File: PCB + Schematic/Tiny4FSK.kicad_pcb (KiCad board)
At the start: 4 copper layers, 35.1 x 73.6 mm, 88 parts, among them J1 Power Ext, J2 GPIO, J3 I2C, J4 USB, J5 USB Breakout, J6 SPI, J7 USBC, J8 SWD, SW1 Power Switch, SW2 RST, U1 BME280, U2 ATGM336H, U3 TPS61200DRC, U4 ECS-327TXO-2012, U5 ATSAMD21G18A-A, U6 SI4063, U7 Linear Step-Down

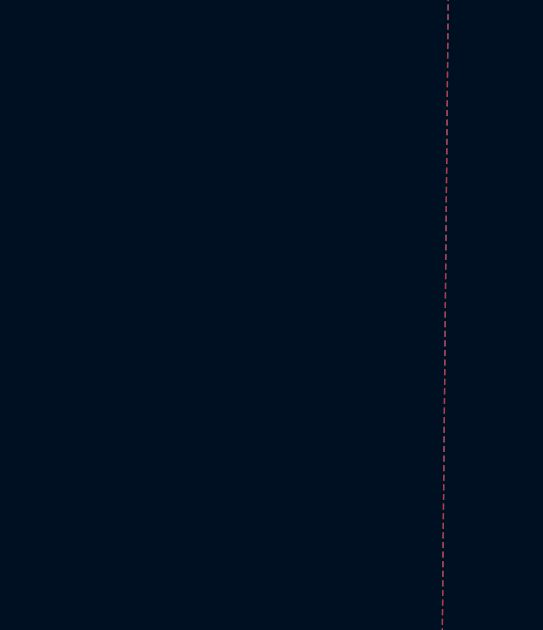
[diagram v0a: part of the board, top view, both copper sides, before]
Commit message: update 3d model paths
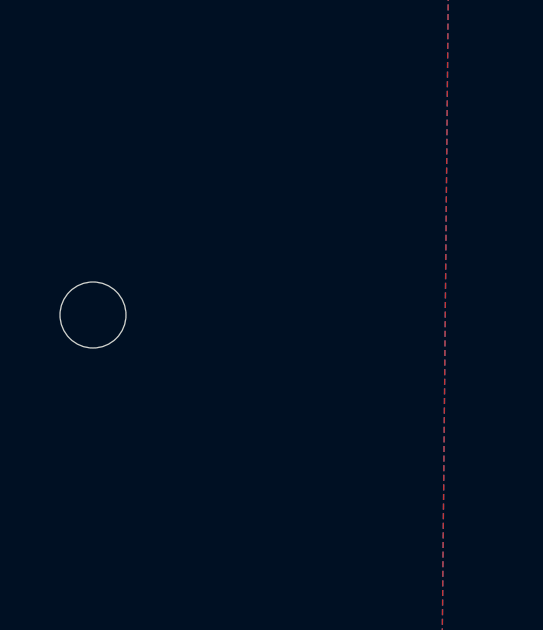
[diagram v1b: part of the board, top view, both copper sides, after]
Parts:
- added H3: MountingHole, MountingHole:MountingHole_2.2mm_M2, F.Cu at (115.0, 64.7)
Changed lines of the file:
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@@
 			(thermal_bridge_angle 45)
 		)
+		(model "${KIPRJMOD}/3D/CM7V-T1A-32.768K-12.5PF-20PPM-TA-QA.step"
+			(offset
+				(xyz 0 0 0)
+			)
+			(scale
+				(xyz 1 1 1)
+			)
+			(rotate
+				(xyz -90 0 0)
+			)
+		)
 	)
 	(footprint "Connector_USB:USB_C_Receptacle_GCT_USB4105-xx-A_16P_TopMnt_Horizontal"
@@
 			(pintype "no_connect")
 		)
-		(model "C:/Users/maxsr/Downloads/User Library-MAX-M8 u-blox M8 Concurrent GNSS Module.step"
+		(model "${KIPRJMOD}/3D/User Library-MAX-M8 u-blox M8 Concurrent GNSS Module.step"
 			(offset
 				(xyz 0 0 0)
@@
 		)
 	)
+	(footprint "MountingHole:MountingHole_2.2mm_M2"
+		(layer "F.Cu")
+		(at 114.975 64.675)
+		(descr "Mounting Hole 2.2mm, no annular, M2")
+		(tags "mounting hole 2.2mm no annular m2")
+		(property "Reference" "H3"
+			(at 0 -3.2 0)
+			(layer "F.SilkS")
+			(hide yes)
+			(effects
+				(font
+					(size 1 1)
+					(thickness 0.15)
+				)
+			)
+		)
+		(property "Value" "MountingHole"
+			(at 0 3.2 0)
+			(layer "F.Fab")
+			(effects
+				(font
+					(size 1 1)
+					(thickness 0.15)
+				)
+			)
+		)
+		(property "Footprint" "MountingHole:MountingHole_2.2mm_M2"
+			(at 0 0 0)
+			(unlocked yes)
+			(layer "F.Fab")
+			(hide yes)
+			(effects
+				(font
+					(size 1.27 1.27)
+					(thickness 0.15)
+				)
+			)
+		)
+		(property "Datasheet" ""
+			(at 0 0 0)
+			(unlocked yes)
+			(layer "F.Fab")
+			(hide yes)
+			(effects
+				(font
+					(size 1.27 1.27)
+					(thickness 0.15)
+				)
+			)
+		)
+		(property "Description" "Mounting Hole without connection"
+			(at 0 0 0)
+			(unlocked yes)
+			(layer "F.Fab")
+			(hide yes)
+			(effects
+				(font
+					(size 1.27 1.27)
+					(thickness 0.15)
+				)
+			)
+		)
+		(property ki_fp_filters "MountingHole*")
+		(sheetname "Root")
+		(sheetfile "Tiny4FSK.kicad_sch")
+		(attr exclude_from_pos_files exclude_from_bom)
+		(fp_circle
+			(center 0 0)
+			(end 2.2 0)
+			(stroke
+				(width 0.15)
+				(type solid)
+			)
+			(fill none)
+			(layer "Cmts.User")
+		)
+		(fp_circle
+			(center 0 0)
+			(end 2.45 0)
+			(stroke
+				(width 0.05)
+				(type solid)
+			)
+			(fill none)
+			(layer "F.CrtYd")
+		)
+		(fp_text user "${REFERENCE}"
+			(at 0 0 0)
+			(layer "F.Fab")
+			(effects
+				(font
+					(size 1 1)
+					(thickness 0.15)
+				)
+			)
+		)
+		(pad "" np_thru_hole circle
+			(at 0 0)
+			(size 2.2 2.2)
+			(drill 2.2)
+			(layers "*.Cu" "*.Mask")
+		)
+	)
 	(footprint "Package_LGA:Bosch_LGA-8_2.5x2.5mm_P0.65mm_ClockwisePinNumbering"
 		(layer "F.Cu")
@@
 			)
 		)
-		(model "C:/Users/maxsr/Downloads/User Library-Bosch_BME280.step"
+		(model "${KIPRJMOD}/3D/shapes3D/shapes3D/User Library-Bosch_BME280.wrl"
 			(offset
 				(xyz 0 0 0)
@@
 			)
 			(rotate
-				(xyz -90 0 0)
+				(xyz -90 0 180)
 			)
 		)
@@
 			(pintype "passive")
 		)
-		(model "C:/Users/maxsr/Downloads/Coilcraft-LPS3015.step"
+		(model "${KIPRJMOD}/3D/Coilcraft-LPS3015.step"
 			(offset
 				(xyz 0 0 0)
@@
 			(thermal_bridge_angle 45)
 		)
+		(model "${KIPRJMOD}/3D/CM7V-T1A-32.768K-12.5PF-20PPM-TA-QA.step"
+			(offset
+				(xyz 0 0 0)
+			)
+			(scale
+				(xyz 1 1 1)
+			)
+			(rotate
+				(xyz -90 0 0)
+			)
+		)
 	)
 	(footprint "Resistor_SMD:R_0402_1005Metric_Pad0.72x0.64mm_HandSolder"
@@
 			)
 		)
-		(model "C:/Users/maxsr/Downloads/1575AT43A0040E/ANT_1575AT_JOT.step"
+		(model "${KIPRJMOD}/3D/ANT_1575AT_JOT.step"
 			(offset
 				(xyz 0 0 0)
